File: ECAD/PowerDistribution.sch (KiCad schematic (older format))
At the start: 8 parts

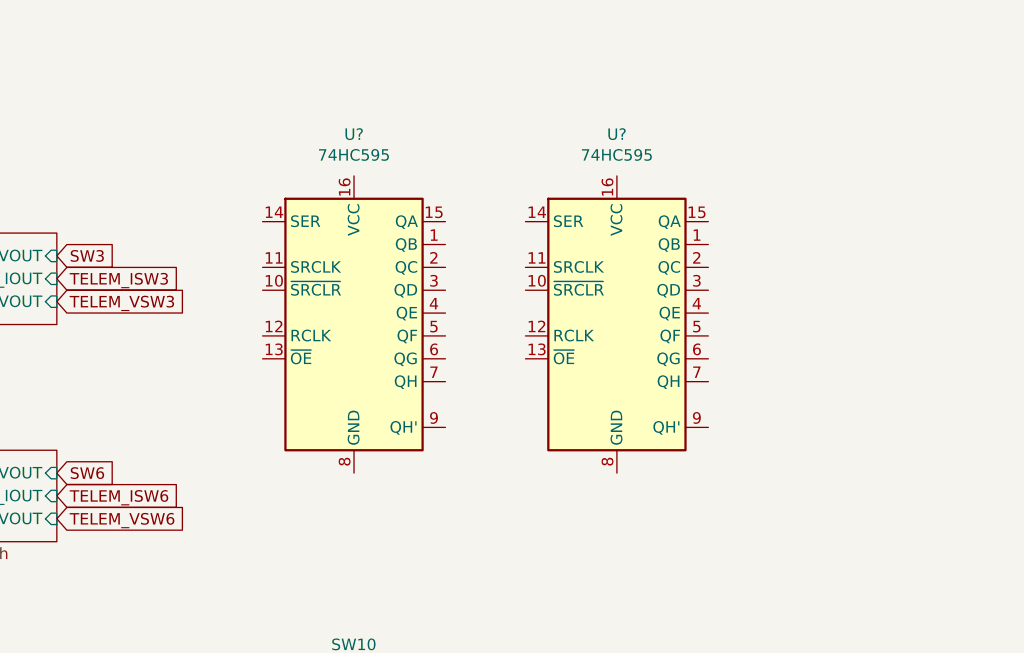
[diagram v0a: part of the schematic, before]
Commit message: Add PDM control using shift registers
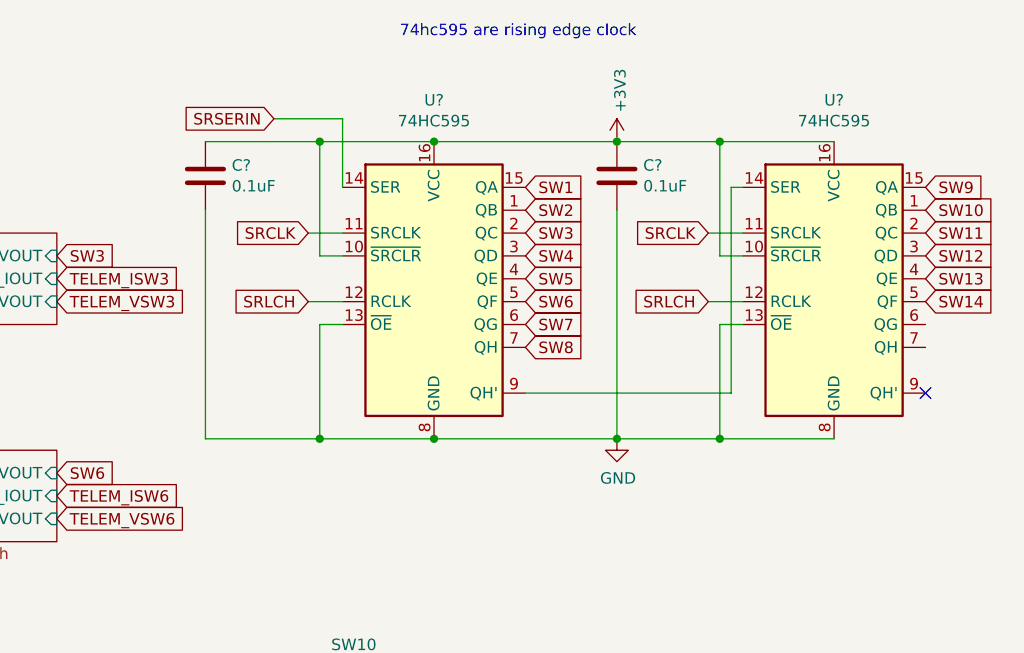
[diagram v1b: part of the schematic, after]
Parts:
- added C? (x2): 0.1uF, symbol Device:C
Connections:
- net +3V3: now also U?.10 (~SRCLR), U?.10 (~SRCLR), U?.16 (VCC), U?.16 (VCC), C?.1, C?.1
- net GND: now also U?.13 (~OE), U?.13 (~OE), U?.8 (GND), U?.8 (GND), C?.2, C?.2
- net SW1: now also U?.15 (QA)
- net SW10: now also U?.1 (QB)
- net SW11: now also U?.2 (QC)
- net SW12: now also U?.3 (QD)
- net SW13: now also U?.4 (QE)
- net SW14: now also U?.5 (QF)
- net SW2: now also U?.1 (QB)
- net SW3: now also U?.2 (QC)
- net SW4: now also U?.3 (QD)
- net SW5: now also U?.4 (QE)
- net SW6: now also U?.5 (QF)
- net SW7: now also U?.6 (QG)
- net SW8: now also U?.7 (QH)
- net SW9: now also U?.15 (QA)
- net SRCLK: now reaches U?.11 (SRCLK)
- net SRCLK: now also U?.11 (SRCLK)
- net SRLCH: now reaches U?.12 (RCLK)
- net SRLCH: now also U?.12 (RCLK)
- net SRSERIN: now reaches U?.14 (SER)
- net at U?.9 (QH'): now also U?.14 (SER)
- no-connect marks 0 -> 1
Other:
- note added: "74hc595 are rising edge clock"
- moved on the sheet: U?
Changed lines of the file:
@@
 L 74xx:74HC595 U?
 U 1 1 622C9B64
-P 8400 1900
-F 0 "U?" H 8400 2681 50  0000 C CNN
-F 1 "74HC595" H 8400 2590 50  0000 C CNN
-F 2 "" H 8400 1900 50  0001 C CNN
-F 3 "http://www.ti.com/lit/ds/symlink/sn74hc595.pdf" H 8400 1900 50  0001 C CNN
-	1    8400 1900
+P 8750 1750
+F 0 "U?" H 8750 2531 50  0000 C CNN
+F 1 "74HC595" H 8750 2440 50  0000 C CNN
+F 2 "" H 8750 1750 50  0001 C CNN
+F 3 "http://www.ti.com/lit/ds/symlink/sn74hc595.pdf" H 8750 1750 50  0001 C CNN
+	1    8750 1750
 	1    0    0    -1
 $EndComp
@@
 L 74xx:74HC595 U?
 U 1 1 622C9F3C
-P 9550 1900
-F 0 "U?" H 9550 2681 50  0000 C CNN
-F 1 "74HC595" H 9550 2590 50  0000 C CNN
-F 2 "" H 9550 1900 50  0001 C CNN
-F 3 "http://www.ti.com/lit/ds/symlink/sn74hc595.pdf" H 9550 1900 50  0001 C CNN
-	1    9550 1900
+P 10500 1750
+F 0 "U?" H 10500 2531 50  0000 C CNN
+F 1 "74HC595" H 10500 2440 50  0000 C CNN
+F 2 "" H 10500 1750 50  0001 C CNN
+F 3 "http://www.ti.com/lit/ds/symlink/sn74hc595.pdf" H 10500 1750 50  0001 C CNN
+	1    10500 1750
 	1    0    0    -1
 $EndComp
@@
 	5400 7300 5200 7300
 Connection ~ 5200 7300
+$Comp
+L power:+3V3 #PWR?
+U 1 1 61DA7D11
+P 9550 1150
+AR Path="/61DA7D11" Ref="#PWR?"  Part="1"
+AR Path="/61BD4B7D/61DA7D11" Ref="#PWR?"  Part="1"
+AR Path="/61E87E93/61DA7D11" Ref="#PWR?"  Part="1"
+F 0 "#PWR?" H 9550 1000 50  0001 C CNN
+F 1 "+3V3" V 9565 1278 50  0000 L CNN
+F 2 "" H 9550 1150 50  0001 C CNN
+F 3 "" H 9550 1150 50  0001 C CNN
+	1    9550 1150
+	1    0    0    -1
+$EndComp
+$Comp
+L power:GND #PWR?
+U 1 1 61DA8643
+P 9550 2450
+AR Path="/61DA8643" Ref="#PWR?"  Part="1"
+AR Path="/61BD4B7D/61DA8643" Ref="#PWR?"  Part="1"
+AR Path="/61E87E93/61DA8643" Ref="#PWR?"  Part="1"
+F 0 "#PWR?" H 9550 2200 50  0001 C CNN
+F 1 "GND" H 9555 2277 50  0000 C CNN
+F 2 "" H 9550 2450 50  0001 C CNN
+F 3 "" H 9550 2450 50  0001 C CNN
+	1    9550 2450
+	1    0    0    -1
+$EndComp
+$Comp
+L Device:C C?
+U 1 1 61DA8C08
+P 9550 1300
+F 0 "C?" H 9665 1346 50  0000 L CNN
+F 1 "0.1uF" H 9665 1255 50  0000 L CNN
+F 2 "" H 9588 1150 50  0001 C CNN
+F 3 "~" H 9550 1300 50  0001 C CNN
+	1    9550 1300
+	1    0    0    -1
+$EndComp
+$Comp
+L Device:C C?
+U 1 1 61DA9C99
+P 7750 1300
+F 0 "C?" H 7865 1346 50  0000 L CNN
+F 1 "0.1uF" H 7865 1255 50  0000 L CNN
+F 2 "" H 7788 1150 50  0001 C CNN
+F 3 "~" H 7750 1300 50  0001 C CNN
+	1    7750 1300
+	1    0    0    -1
+$EndComp
+Wire Wire Line
+	10500 1150 10000 1150
+Connection ~ 8750 1150
+Wire Wire Line
+	8750 1150 8250 1150
+Wire Wire Line
+	7750 1450 7750 2450
+Wire Wire Line
+	8750 2450 9550 2450
+Connection ~ 8750 2450
+Wire Wire Line
+	8350 1650 8250 1650
+Wire Wire Line
+	8250 1650 8250 1150
+Connection ~ 8250 1150
+Wire Wire Line
+	10100 1650 10000 1650
+Wire Wire Line
+	10000 1650 10000 1150
+Connection ~ 10000 1150
+Wire Wire Line
+	8350 1950 8250 1950
+Text Notes 8600 700  0    50   ~ 0
+74hc595 are rising edge clock
+Wire Wire Line
+	10050 1350 10050 2250
+Wire Wire Line
+	10100 1950 10000 1950
+Wire Wire Line
+	10000 1950 10000 2450
+Connection ~ 10000 2450
+Wire Wire Line
+	10000 2450 10500 2450
+Wire Wire Line
+	8250 1950 8250 2450
+Connection ~ 8250 2450
+Wire Wire Line
+	8250 2450 8750 2450
+Wire Wire Line
+	10050 1350 10100 1350
+Wire Wire Line
+	9150 2250 10050 2250
+Wire Wire Line
+	8350 1350 8350 1050
+Wire Wire Line
+	8350 1050 8050 1050
+Wire Wire Line
+	8350 1850 8200 1850
+Wire Wire Line
+	8350 1550 8200 1550
+Wire Wire Line
+	10100 1550 9950 1550
+Wire Wire Line
+	10100 1850 9950 1850
+Text GLabel 8200 1550 0    50   Input ~ 0
+SRCLK
+Text GLabel 9950 1550 0    50   Input ~ 0
+SRCLK
+Text GLabel 8200 1850 0    50   Input ~ 0
+SRLCH
+Text GLabel 9950 1850 0    50   Input ~ 0
+SRLCH
+Text GLabel 8050 1050 0    50   Input ~ 0
+SRSERIN
+Text GLabel 9150 1350 2    50   Input ~ 0
+SW1
+Text GLabel 9150 1450 2    50   Input ~ 0
+SW2
+Text GLabel 9150 1550 2    50   Input ~ 0
+SW3
+Text GLabel 9150 1650 2    50   Input ~ 0
+SW4
+Text GLabel 9150 1750 2    50   Input ~ 0
+SW5
+Text GLabel 9150 1850 2    50   Input ~ 0
+SW6
+Text GLabel 9150 1950 2    50   Input ~ 0
+SW7
+Text GLabel 9150 2050 2    50   Input ~ 0
+SW8
+Text GLabel 10900 1350 2    50   Input ~ 0
+SW9
+Text GLabel 10900 1450 2    50   Input ~ 0
+SW10
+Text GLabel 10900 1550 2    50   Input ~ 0
+SW11
+Text GLabel 10900 1650 2    50   Input ~ 0
+SW12
+Text GLabel 10900 1750 2    50   Input ~ 0
+SW13
+Text GLabel 10900 1850 2    50   Input ~ 0
+SW14
+Connection ~ 9550 1150
+Wire Wire Line
+	9550 1150 8750 1150
+Connection ~ 9550 2450
+Wire Wire Line
+	9550 2450 10000 2450
+Wire Wire Line
+	9550 1450 9550 2450
+Wire Wire Line
+	9550 1150 10000 1150
+NoConn ~ 10900 2250
+Wire Wire Line
+	7750 1150 8250 1150
+Wire Wire Line
+	7750 2450 8250 2450
 $EndSCHEMATC
